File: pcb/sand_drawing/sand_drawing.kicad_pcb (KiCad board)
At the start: 2 copper layers, 54.2 x 89.3 mm, 38 parts, among them J0 12V GND, J1 Stepper1, J2 Stepper2, J3 Opto 1, J4 Opto 2, J5 UART, SW1 EN, SW2 IO0, U2 AMS1117-3.3, U3 ESP32-WROOM-32D

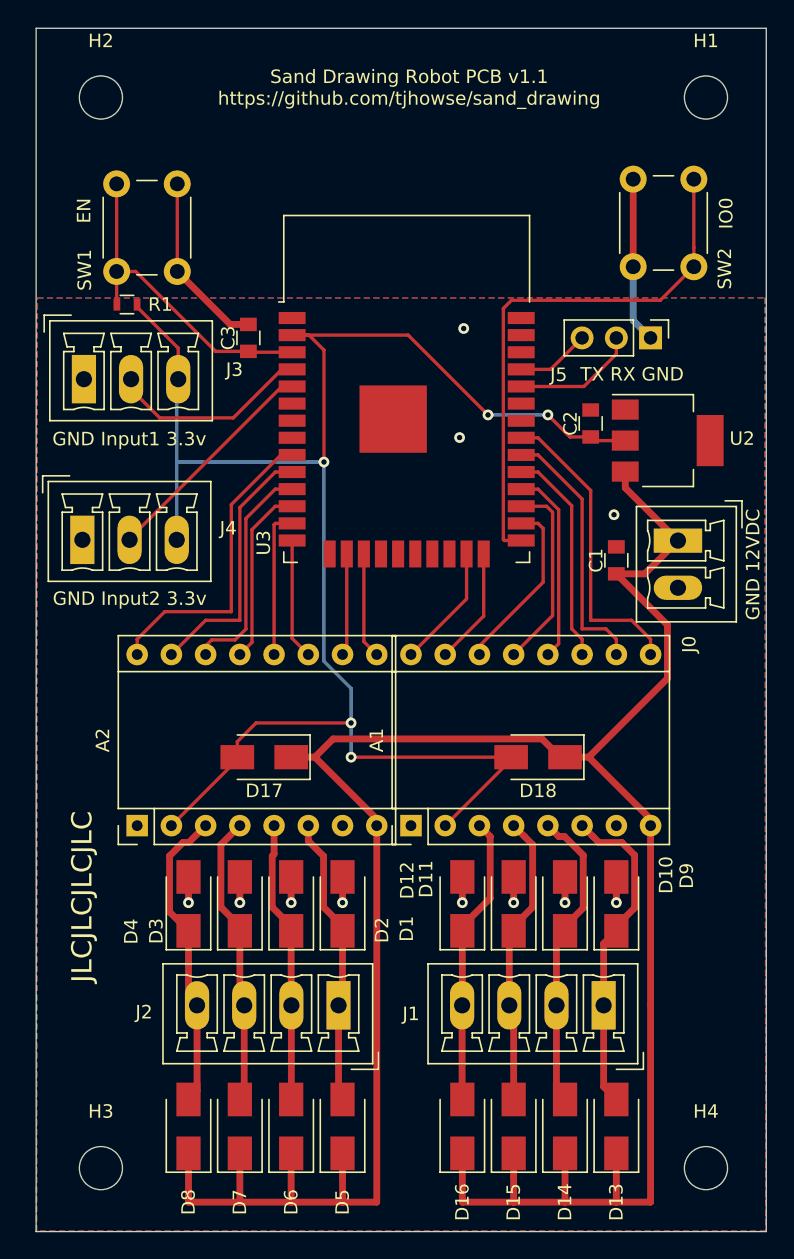
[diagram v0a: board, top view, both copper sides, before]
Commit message: v1.1 of the PCB nearly done.
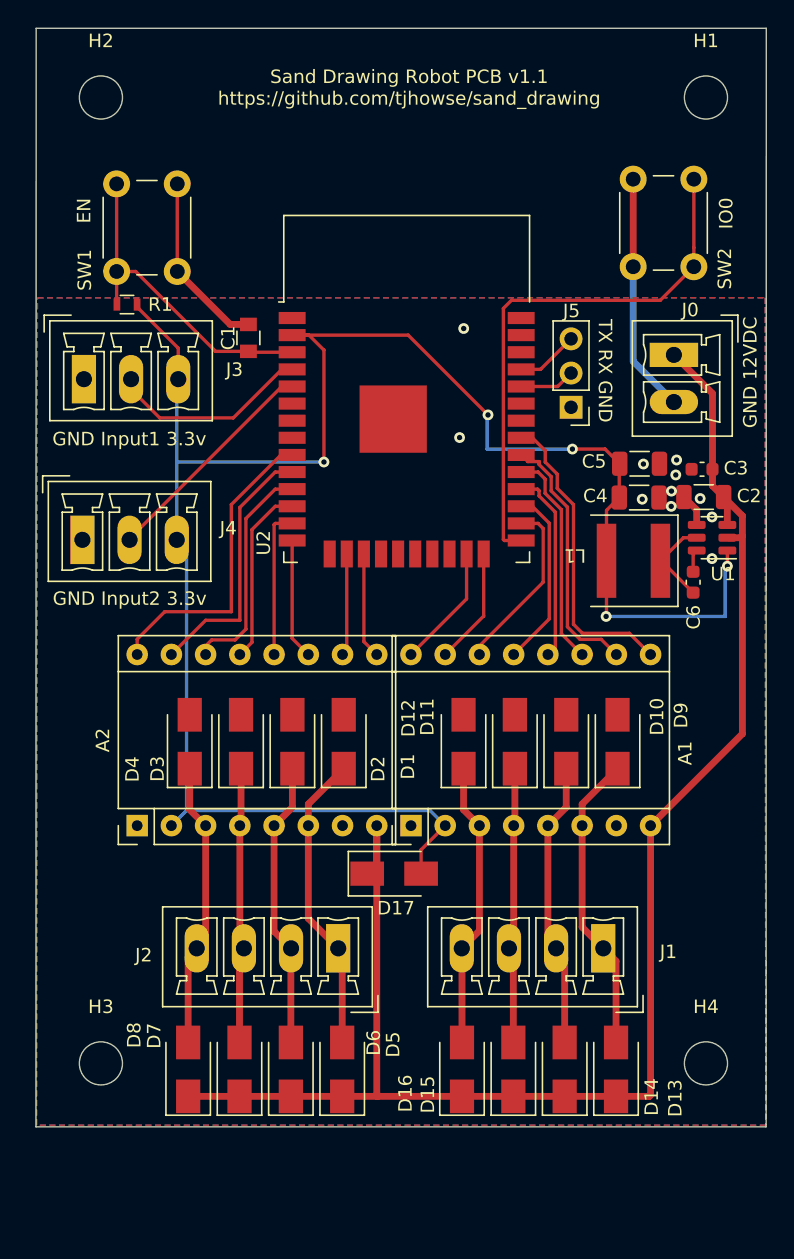
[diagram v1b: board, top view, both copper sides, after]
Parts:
- removed D18: SS210 Schottky Diode, Diode_SMD:D_SMA
- removed the U2 at (143.5, 105.4)
- added C3: 100nF/50V, Capacitor_SMD:C_0603_1608Metric, F.Cu at (146.1, 107.5)
- added C5: 22µF/25V, Capacitor_SMD:C_1206_3216Metric, F.Cu at (141.4, 107.1)
- added C6: 100nF/50V, Capacitor_SMD:C_0603_1608Metric, F.Cu at (145.4, 115.9)
- added L1: 6.8µH, sand_drawing_parts:WURTH_6060, F.Cu at (141.0, 114.3)
- added U1: AP63203WU, Package_TO_SOT_SMD:TSOT-23-6, F.Cu at (146.8, 112.6)
- C2: renamed from C1; value 10µF/25V -> 10µF/35V; footprint Capacitors_SMD:C_0805 -> Capacitor_SMD:C_1206_3216Metric
- C4: renamed from C2; value 10µF/25V -> 22µF/25V; footprint Capacitors_SMD:C_0805 -> Capacitor_SMD:C_1206_3216Metric
- moved J0 13.8 mm to (144.0, 99.0)
- moved D17 12.9 mm to (123.2, 137.6), turned to 0 degrees
- moved D1 12.0 mm to (119.5, 127.8)
- moved D10 12.0 mm to (136.0, 127.8)
- moved D11 12.0 mm to (132.2, 127.8)
- moved D12 12.0 mm to (128.4, 127.8)
- moved D2 12.0 mm to (115.7, 127.8)
- moved D3 12.0 mm to (111.8, 127.8)
- moved D4 12.0 mm to (108.0, 127.8)
- moved D9 12.0 mm to (139.8, 127.8)
- moved C2 8.01 mm to (146.2, 109.6), turned to 180 degrees
- moved J5 7.83 mm to (136.3, 102.9), turned to 180 degrees
- moved H3 7.77 mm to (101.5, 151.6)
- moved H4 7.77 mm to (146.3, 151.6)
- moved C4 6.57 mm to (141.4, 109.6), turned to 0 degrees
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- renumbered C3 to C1, U3 to U2
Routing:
- net +12V: track 179.9 -> 121.5 mm
- net +3V3: track 127.6 -> 142.0 mm
- net GND: track 41.0 -> 33.7 mm
- net Net-(C6-Pad1): track 0.00 -> 6.81 mm
- net RX: track 9.26 -> 4.11 mm
- net Net-(A1-Pad6): track 24.3 -> 22.4 mm
- net Net-(C6-Pad2): track 0.00 -> 1.68 mm
- net Net-(A2-Pad3): track 22.8 -> 21.3 mm
- net Net-(A1-Pad5): track 22.7 -> 21.4 mm
- net Net-(A2-Pad4): track 21.8 -> 20.6 mm
- net Net-(A1-Pad4): track 21.8 -> 20.6 mm
- net TX: track 5.49 -> 4.64 mm
- net Net-(A2-Pad6): track 21.6 -> 22.4 mm
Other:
- board size 54.2 x 89.3 mm -> 54.2 x 81.5 mm
- board text removed: "JLCJLCJLCJLC"
